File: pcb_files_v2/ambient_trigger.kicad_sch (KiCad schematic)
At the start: 31 parts, among them K1 G5Q-1, Q14 2N3904, U2 4069, U5 4040, U8 555(NEW_layout)

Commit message: updated 555 footprint, it was too big
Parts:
- U8: footprint Package_SO:SOIC-8_5.275x5.275mm_P1.27mm -> Package_SO:SOIC-8_3.9x4.9mm_P1.27mm
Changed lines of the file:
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@@
       (effects (font (size 1.27 1.27)) (justify left))
     )
-    (property "Footprint" "Package_SO:SOIC-8_5.275x5.275mm_P1.27mm" (id 2) (at 157.48 129.54 0)
+    (property "Footprint" "Package_SO:SOIC-8_3.9x4.9mm_P1.27mm" (id 2) (at 157.48 129.54 0)
       (effects (font (size 1.27 1.27)) hide)
     )

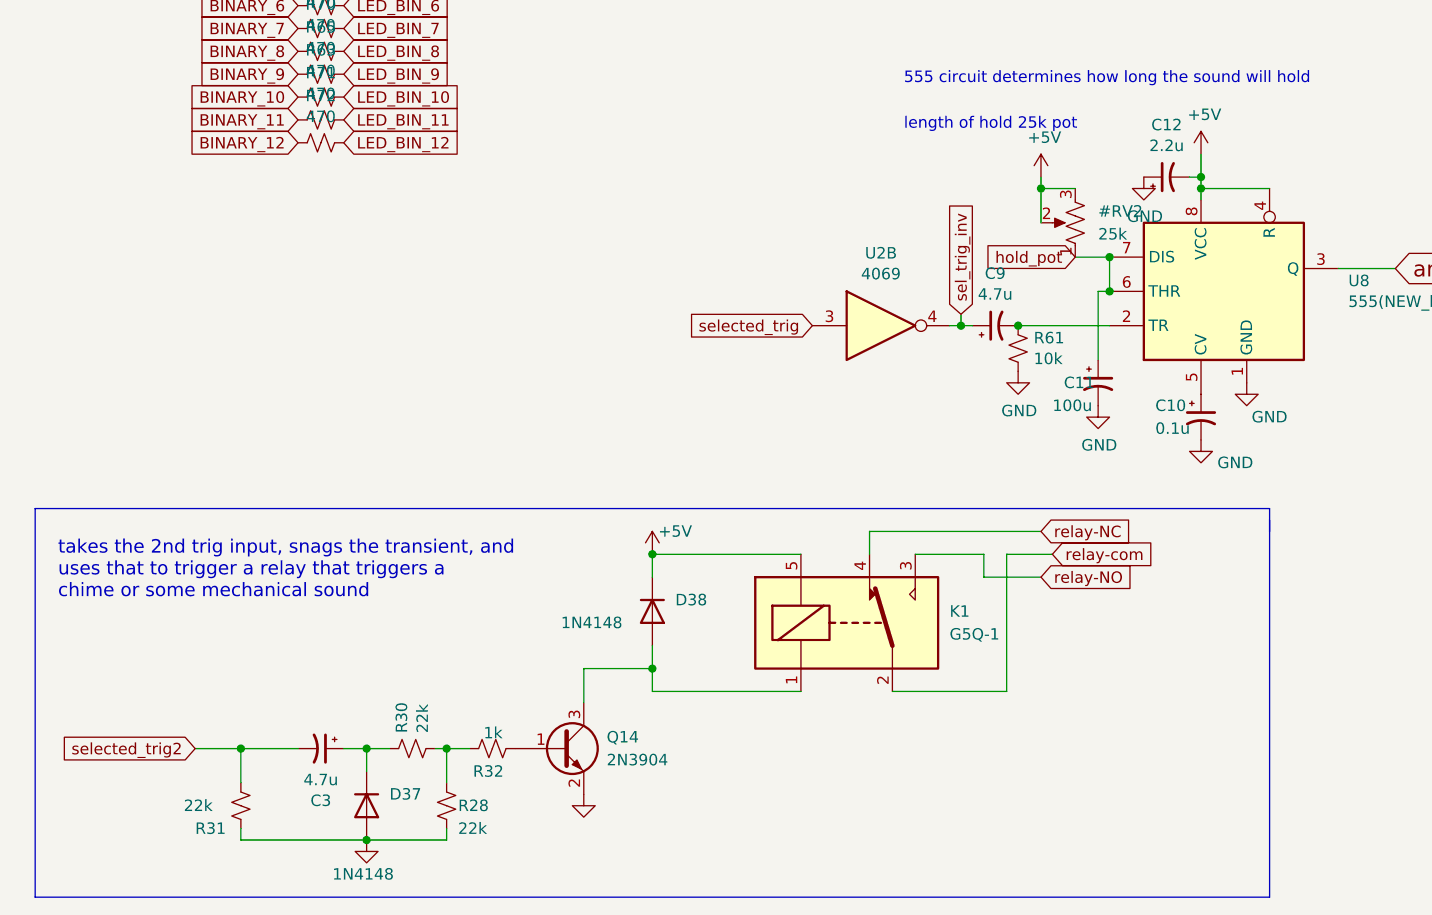
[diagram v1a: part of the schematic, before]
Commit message: oct 2025 update
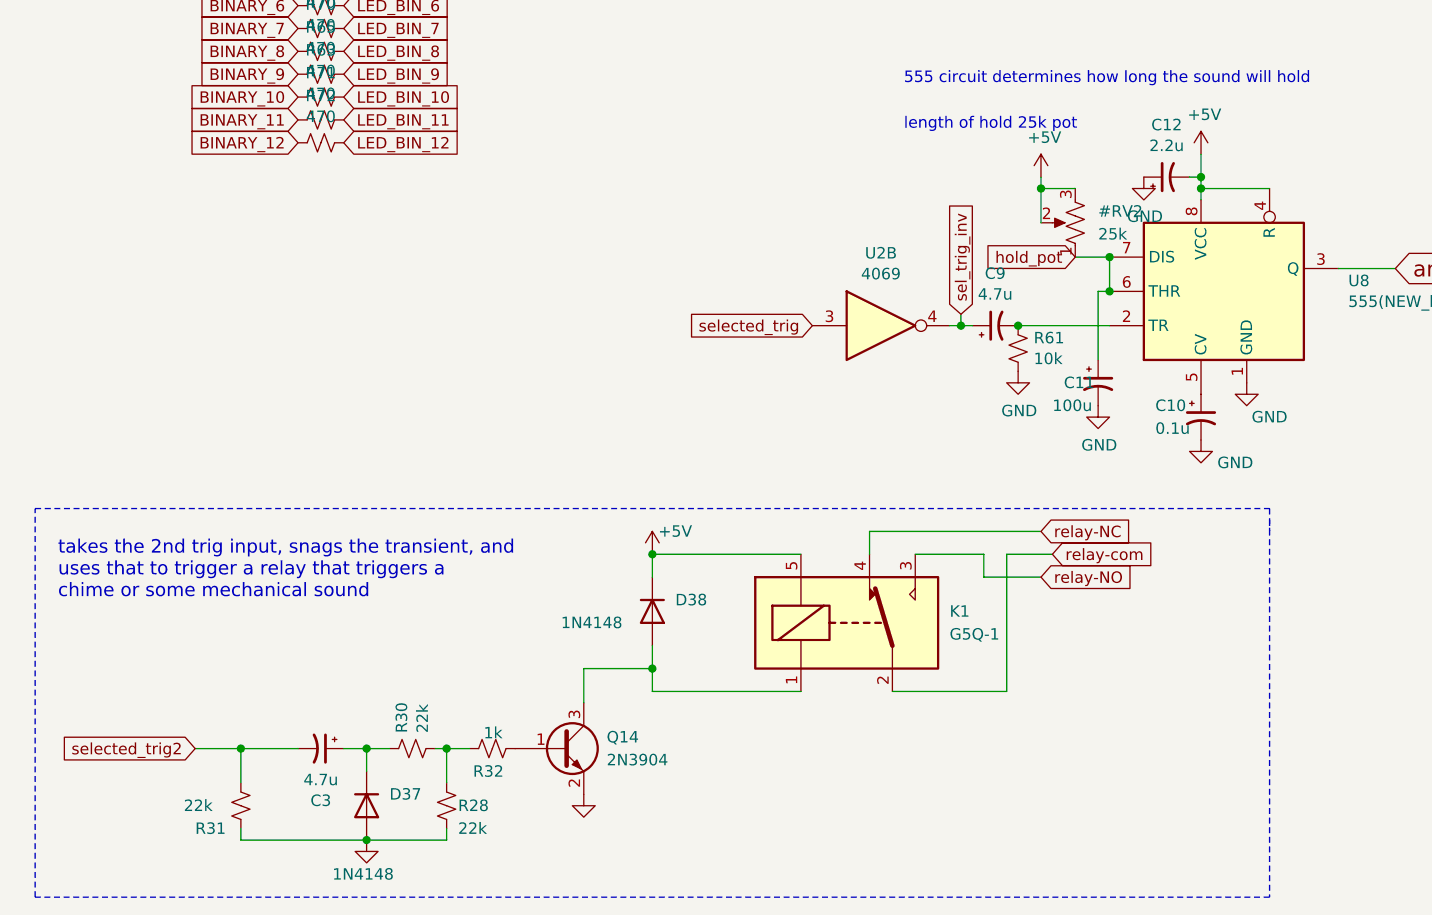
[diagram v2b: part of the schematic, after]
